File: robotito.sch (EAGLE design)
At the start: 54 parts, among them IC1 7805T, IC2 L298, IC3 L298, J1 22-27-2031-03, J10 22-27-2031-03, J11 22-27-2031-03, J12 22-27-2031-03, J2 22-27-2031-03, J3 22-27-2031-03, J4 22-27-2031-03, J5 22-27-2031-03, J6 22-27-2031-03, J7 22-27-2031-03, J8 22-27-2031-03, J9 22-27-2031-03

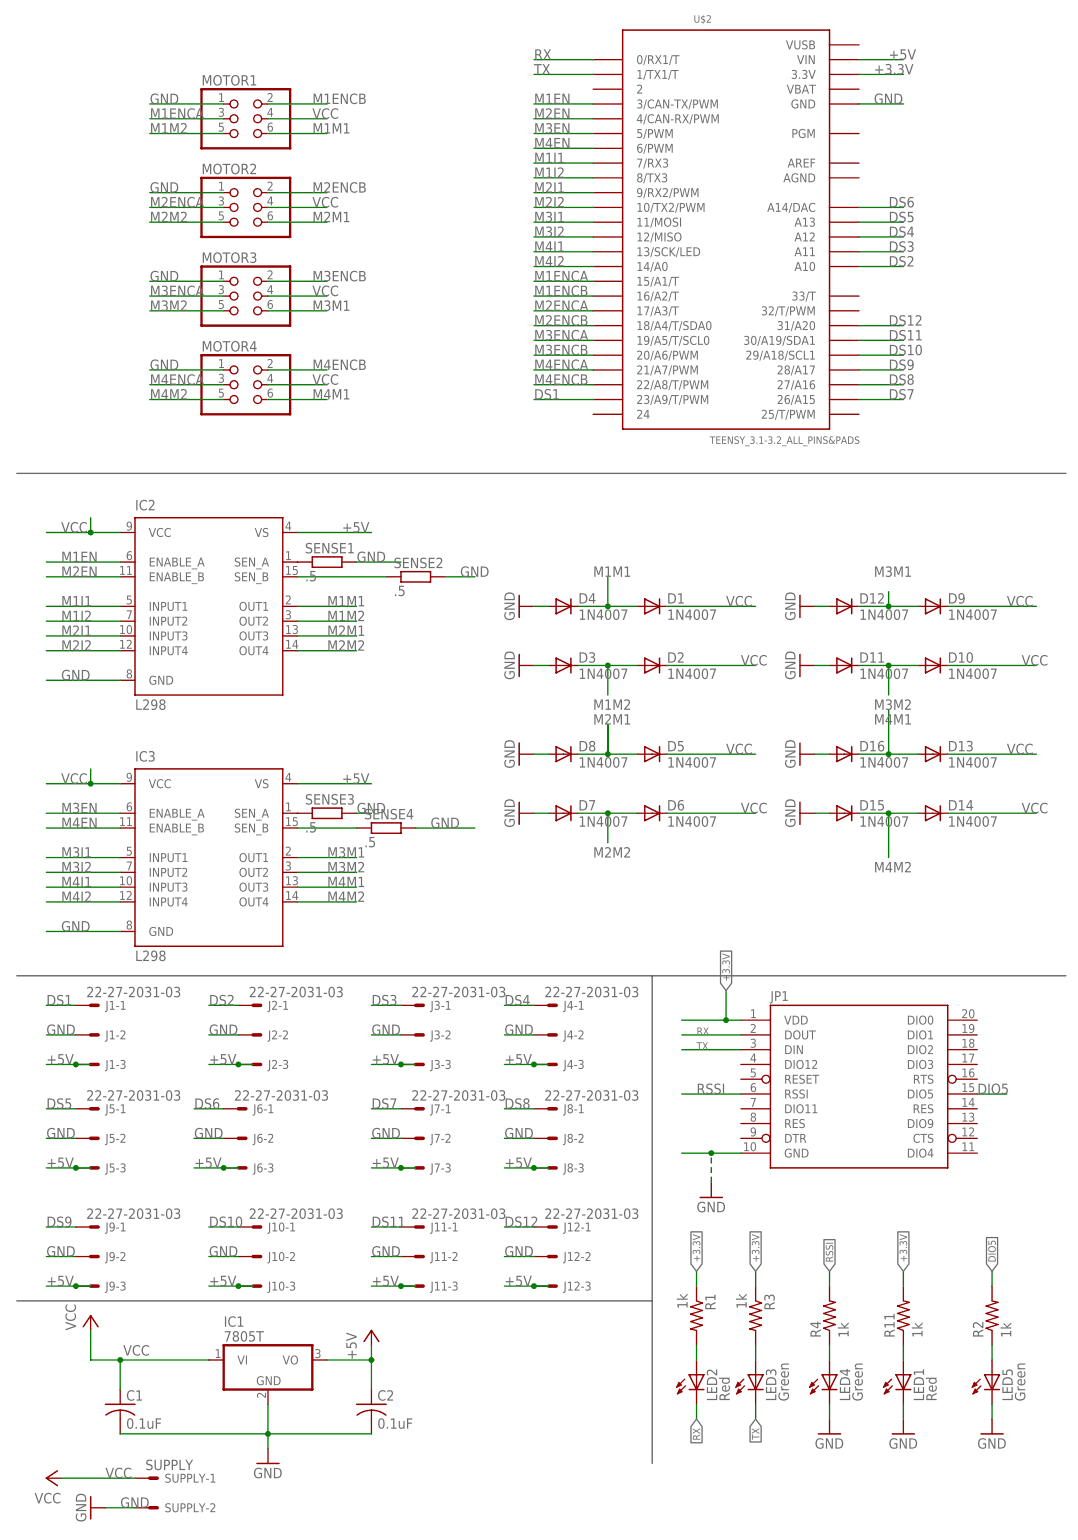
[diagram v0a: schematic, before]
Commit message: juan and tj improvements draft
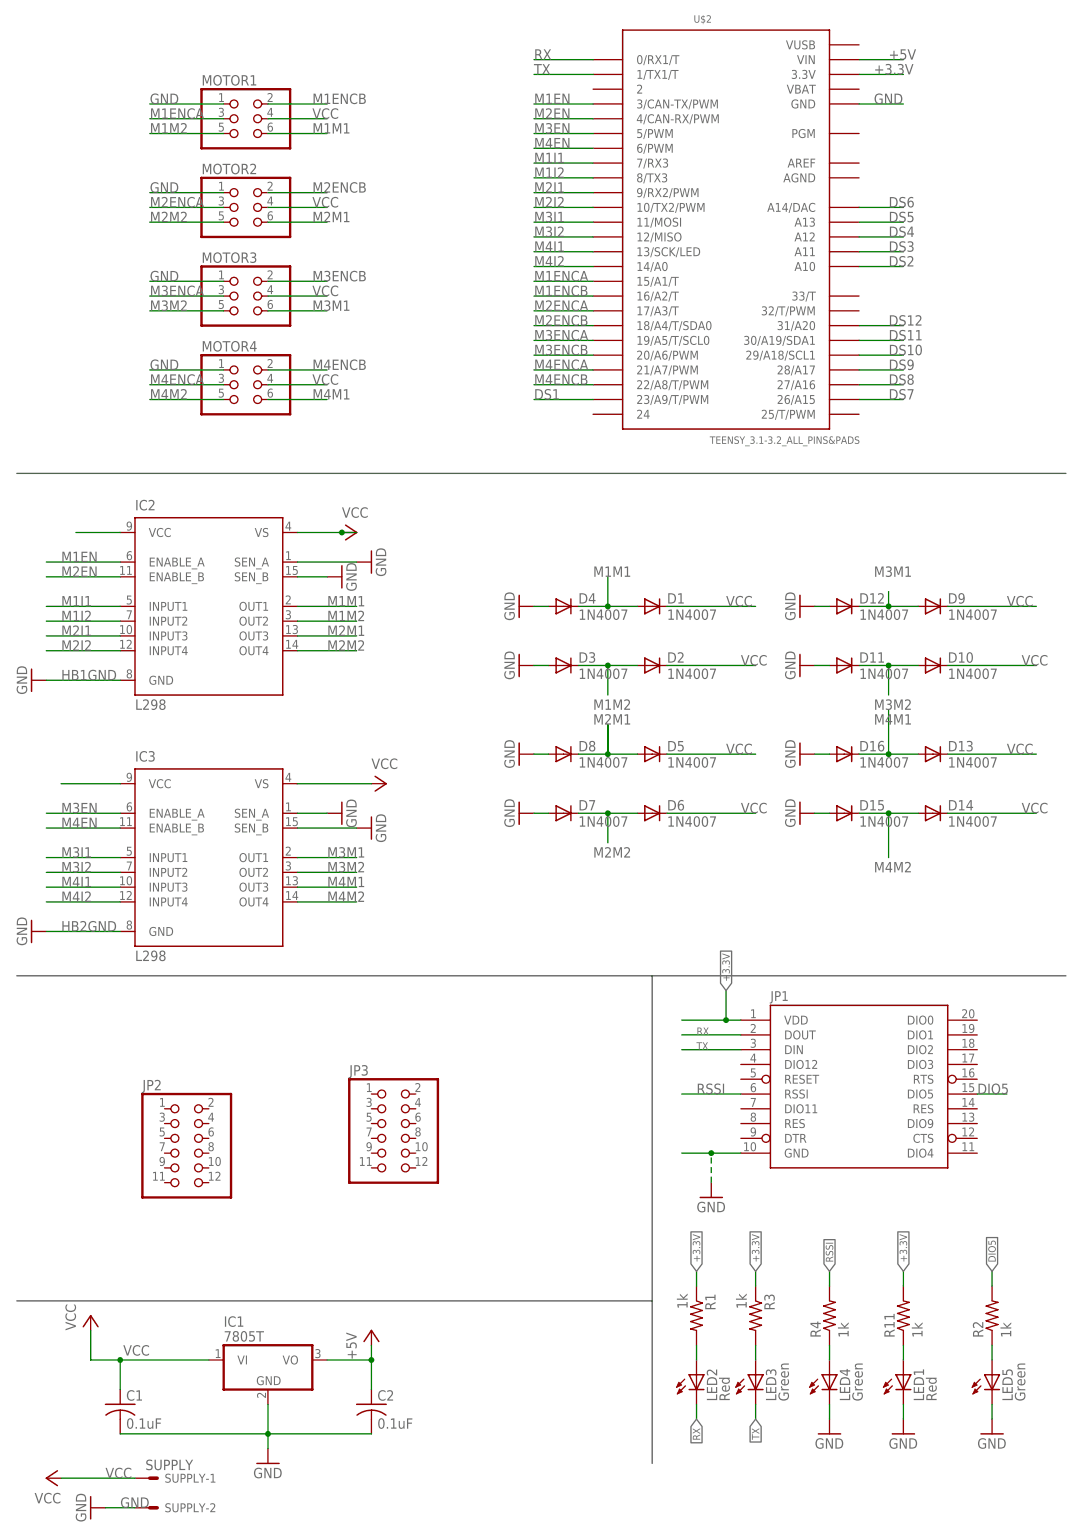
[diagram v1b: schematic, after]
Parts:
- removed J1, J10, J11, J12, J2, J3, J4, J5, J6, J7, J8, J9: 22-27-2031-03, con-molex:22-27-2031-03
- removed SENSE1, SENSE2, SENSE3, SENSE4: .5, resistor:R-EU_0204/7
- added JP2, JP3: (no value), pinhead:PINHD-2X6
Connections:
- removed net N$10: IC2.SEN_A, SENSE1.1
- removed net N$11: IC2.SEN_B, SENSE2.1
- removed net N$3: IC3.SEN_A, SENSE3.1
- removed net N$8: IC3.SEN_B, SENSE4.1
- new net HB1GND: IC2.GND
- new net HB2GND: IC3.GND
- net +5V: now also IC2.VCC, IC3.VCC; no longer IC2.VS, IC3.VS, J1-3.S, J10-3.S, J11-3.S, J12-3.S, J2-3.S, J3-3.S, J4-3.S, J5-3.S, J6-3.S, J7-3.S, J8-3.S, J9-3.S
- net DS1: no longer J1-1.S
- net DS10: no longer J10-1.S
- net DS11: no longer J11-1.S
- net DS12: no longer J12-1.S
- net DS2: no longer J2-1.S
- net DS3: no longer J3-1.S
- net DS4: no longer J4-1.S
- net DS5: no longer J5-1.S
- net DS6: no longer J6-1.S
- net DS7: no longer J7-1.S
- net DS8: no longer J8-1.S
- net DS9: no longer J9-1.S
- net GND: now also IC2.SEN_A, IC2.SEN_B, IC3.SEN_A, IC3.SEN_B; no longer IC2.GND, IC3.GND, J1-2.S, J10-2.S, J11-2.S, J12-2.S, J2-2.S, J3-2.S, J4-2.S, J5-2.S, J6-2.S, J7-2.S, J8-2.S, J9-2.S, SENSE1.2, SENSE2.2, SENSE3.2, SENSE4.2
- net VCC: now also IC2.VS, IC3.VS; no longer IC2.VCC, IC3.VCC
